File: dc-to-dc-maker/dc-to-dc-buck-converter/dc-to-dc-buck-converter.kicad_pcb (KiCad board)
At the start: 2 copper layers, 100 x 80 mm, 33 parts, among them IC1 LA_55-P, IC2 LA_55-P, IC3 EL7104CNZ, J1 Conn_01x06_Pin, J2 Jgen, J3 Jaux 9V, J4 Jind, J5 Jout +50V, U1 IRF640NPBF

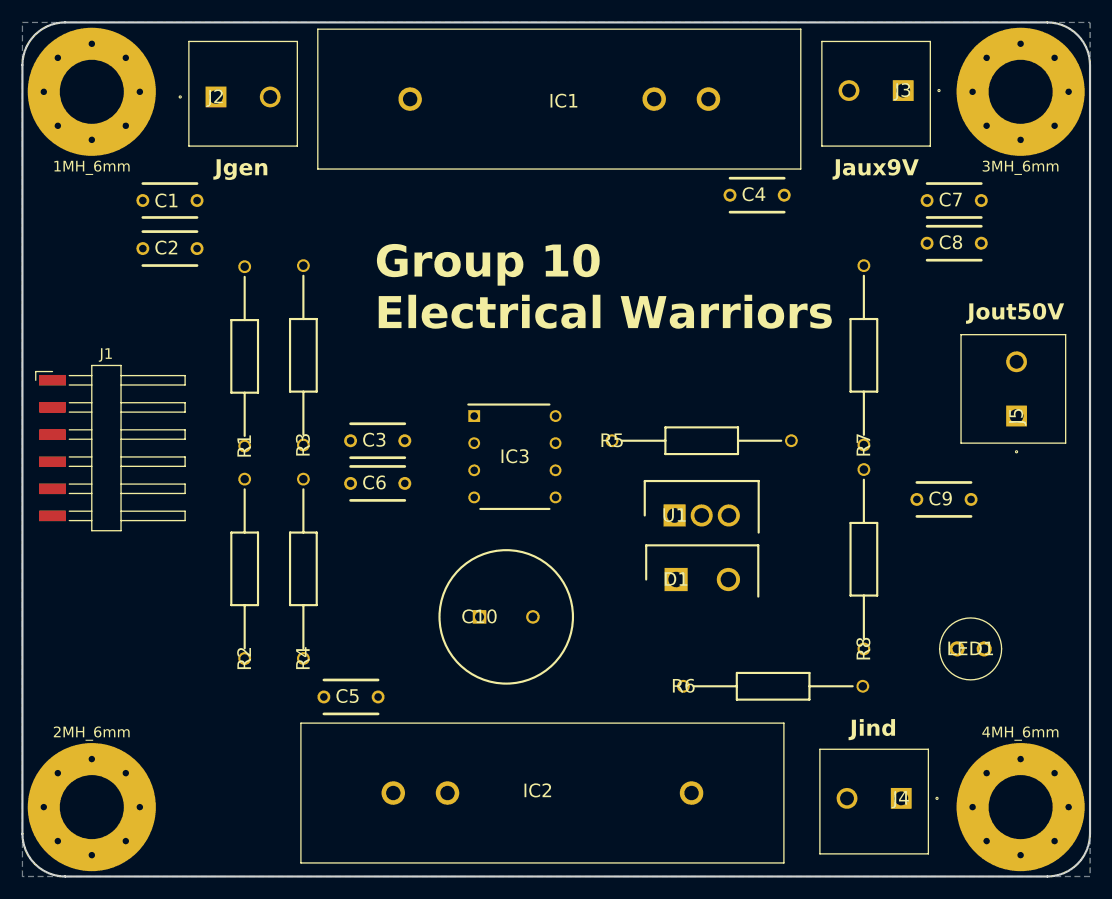
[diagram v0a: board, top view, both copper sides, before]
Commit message: pcb final
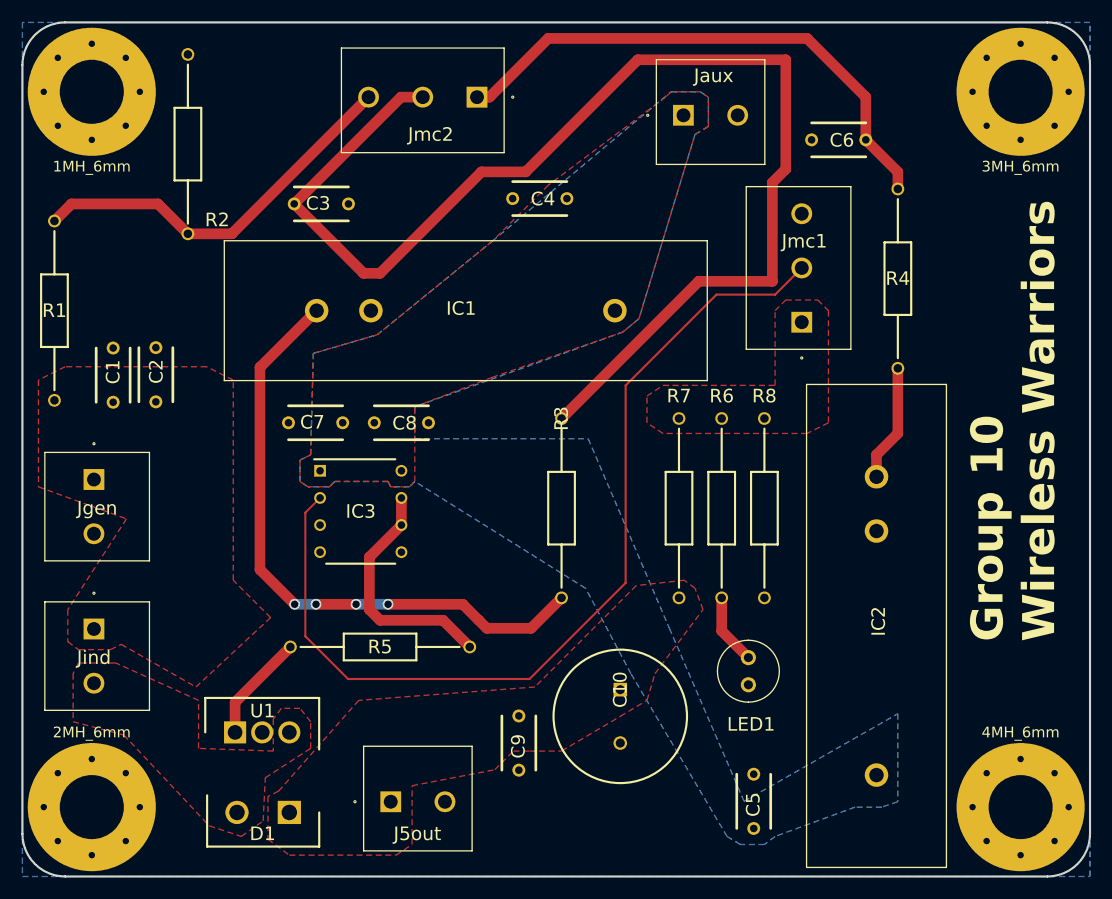
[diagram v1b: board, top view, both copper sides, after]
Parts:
- removed J1: Conn_01x06_Pin, Connector_Harwin:Harwin_M20-89006xx_1x06_P2.54mm_Horizontal
- added Jmc1: 1715734, 1715734(screw connector):1715734, F.Cu at (173.0, 78.1)
- added Jmc2: 1715734, 1715734(screw connector):1715734, F.Cu at (142.6, 57.0)
- Jaux: renamed from J3; value Jaux 9V -> Jaux
- moved Jind 77.3 mm to (106.7, 106.8), turned to -90 degrees
- moved R4 71.0 mm to (182.0, 65.6), turned to -90 degrees
- moved J5out 68.9 mm to (134.5, 123.0), turned to 0 degrees
- moved C7 63.3 mm to (127.5, 87.5)
- moved R2 56.8 mm to (115.5, 53.0), turned to -90 degrees
- moved C8 54.4 mm to (135.5, 87.5), turned to 180 degrees
- moved C6 53.9 mm to (176.5, 61.0), turned to 180 degrees
- moved U1 45.9 mm to (119.9, 116.5)
- moved C9 45.9 mm to (146.5, 117.5), turned to 90 degrees
- moved D1 42.3 mm to (125.0, 124.0), turned to 180 degrees
- moved C5 39.0 mm to (168.5, 123.0), turned to 90 degrees
- moved Jgen 37.6 mm to (106.7, 92.8), turned to -90 degrees
- moved R1 27.6 mm to (103.0, 68.6), turned to -90 degrees
- moved IC1 27.6 mm to (155.5, 77.0), turned to 0 degrees
- moved R6 25.3 mm to (165.5, 87.1), turned to -90 degrees
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- renumbered J5 to J5out, J2 to Jgen, J4 to Jind
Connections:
- C5 pad 1: Net-(IC2-POS) -> Net-(IC1-POS)
- IC2 pad 3: Net-(IC2-POS) -> Net-(IC1-POS)
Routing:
- net Net-(C3-Pad1): track 0.00 -> 119.5 mm
- net Net-(IC3-IN): track 0.00 -> 88.5 mm
- net Net-(IC1-M): track 0.00 -> 58.2 mm, vias 0 -> 4
- net Net-(C6-Pad1): track 0.00 -> 50.8 mm
- net Net-(Jmc2-Pad3): track 0.00 -> 36.5 mm
- net Net-(IC3-N_OUT): track 0.00 -> 22.6 mm
- net Net-(IC2-M): track 0.00 -> 11.0 mm
- net Net-(U1-GATE): track 0.00 -> 10.1 mm
- net Net-(LED1-A): track 0.00 -> 6.64 mm
- added copper zone on F.Cu, net Net-(C1-Pad2)
- added copper zone on F.Cu, net Net-(C10-+)
- added copper zone on F.Cu, net Net-(D1-A)
- added copper zone on B.Cu, net Net-(IC1-POS)
- added copper zone on F.Cu, net Net-(IC1-POS)
- added copper zone on F.Cu, net Net-(Jmc1-Pad1)
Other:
- board text added: "Group 10 Wireless Warriors"
- board text removed: "Group 10 Electrical Warriors"
- board text removed: "Jaux9V"
- board text removed: "Jgen"
- board text removed: "Jind"
- board text removed: "Jout50V"
